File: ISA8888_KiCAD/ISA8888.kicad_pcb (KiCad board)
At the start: 2 copper layers, 59 parts, among them J1 Bus_PCI_32bit_Universal, J2 Bus_ISA_16bit, J3 Conn_02x03, J4 Conn_02x02, U2 AT24CS02-SSHM, Y1 CFPS-72

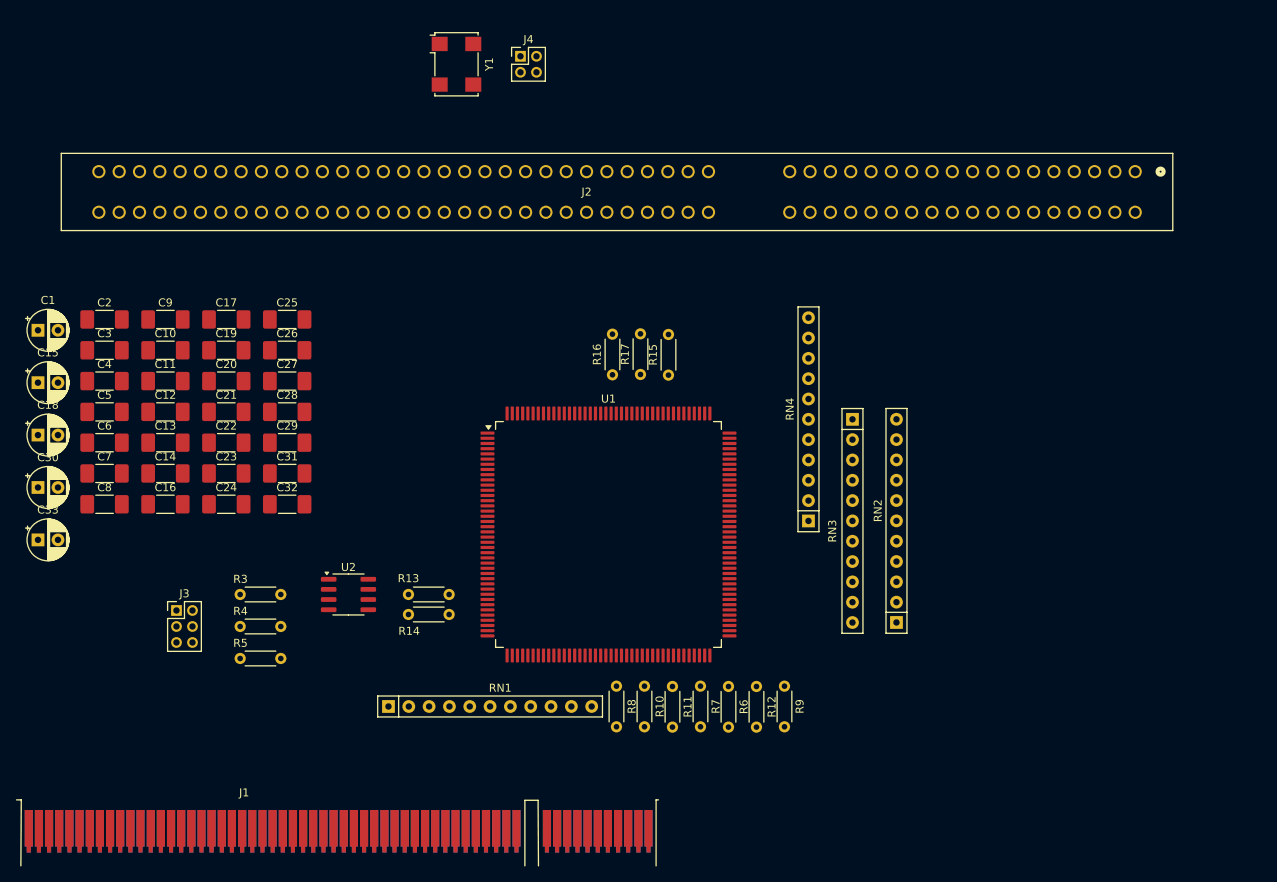
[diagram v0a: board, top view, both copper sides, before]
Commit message: Temp
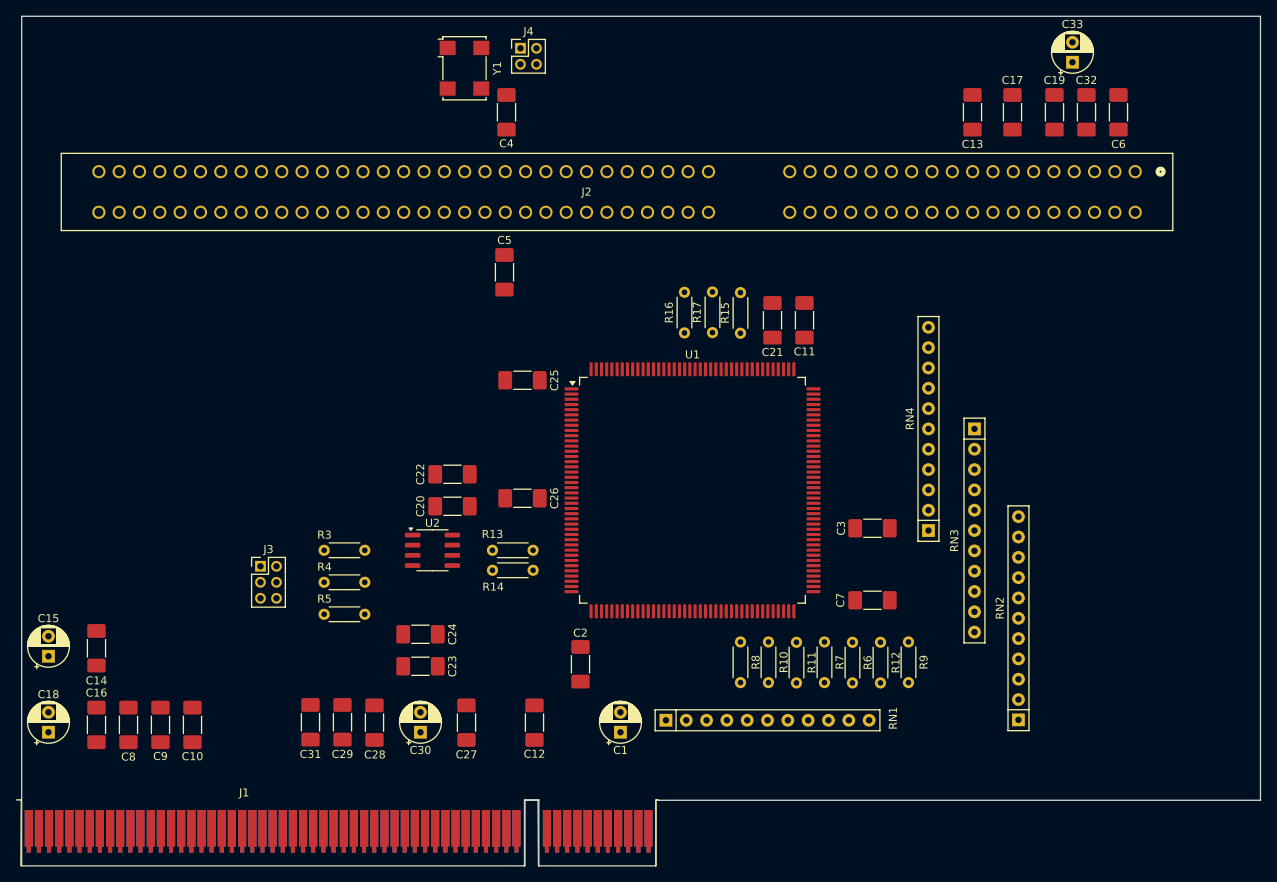
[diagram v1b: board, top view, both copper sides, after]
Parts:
- moved C33 142.4 mm to (211.5, 43.8), turned to 90 degrees
- moved C6 133.3 mm to (217.2, 50.0), turned to 90 degrees
- moved C32 111.3 mm to (213.2, 50.0), turned to 90 degrees
- moved C13 109.0 mm to (199.0, 50.0), turned to 90 degrees
- moved C19 107.7 mm to (209.2, 50.0), turned to 90 degrees
- moved C17 101.6 mm to (204.0, 50.0), turned to 90 degrees
- moved C3 98.5 mm to (186.5, 102.0)
- moved C7 97.3 mm to (186.5, 111.0)
- moved C1 88.5 mm to (155.0, 127.5), turned to 90 degrees
- moved C11 80.2 mm to (178.0, 76.0), turned to 90 degrees
- moved C2 73.5 mm to (150.0, 119.0), turned to -90 degrees
- moved C21 69.2 mm to (174.0, 76.0), turned to 90 degrees
- moved C4 60.4 mm to (140.8, 50.0), turned to 90 degrees
- moved C12 60.3 mm to (144.2, 126.3), turned to 90 degrees
- moved C30 56.8 mm to (130.0, 127.5), turned to 90 degrees
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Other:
- board outline added: 154.8 x 106.2 mm
